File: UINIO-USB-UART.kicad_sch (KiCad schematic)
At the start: 32 parts, among them J1 Conn_01x08_Male, J2 Conn_01x04_Male, J3 Conn_01x07_Male, J4 Conn_01x06_Male, J5 Conn_01x04_Male, J6 Conn_01x07_Male, SW1 TP-33103, U1 CP2102, U2 CH343P

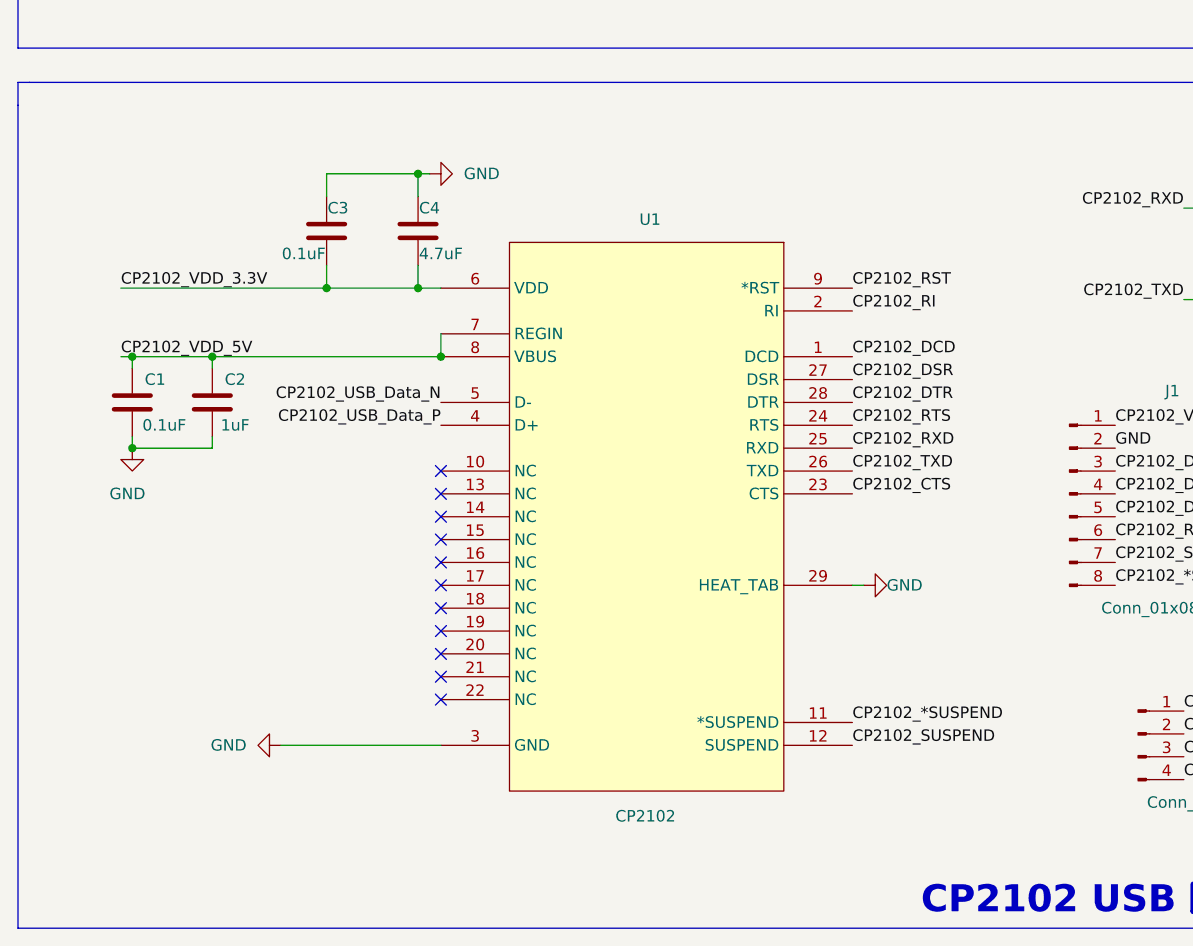
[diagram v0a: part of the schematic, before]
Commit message: Update libraries.
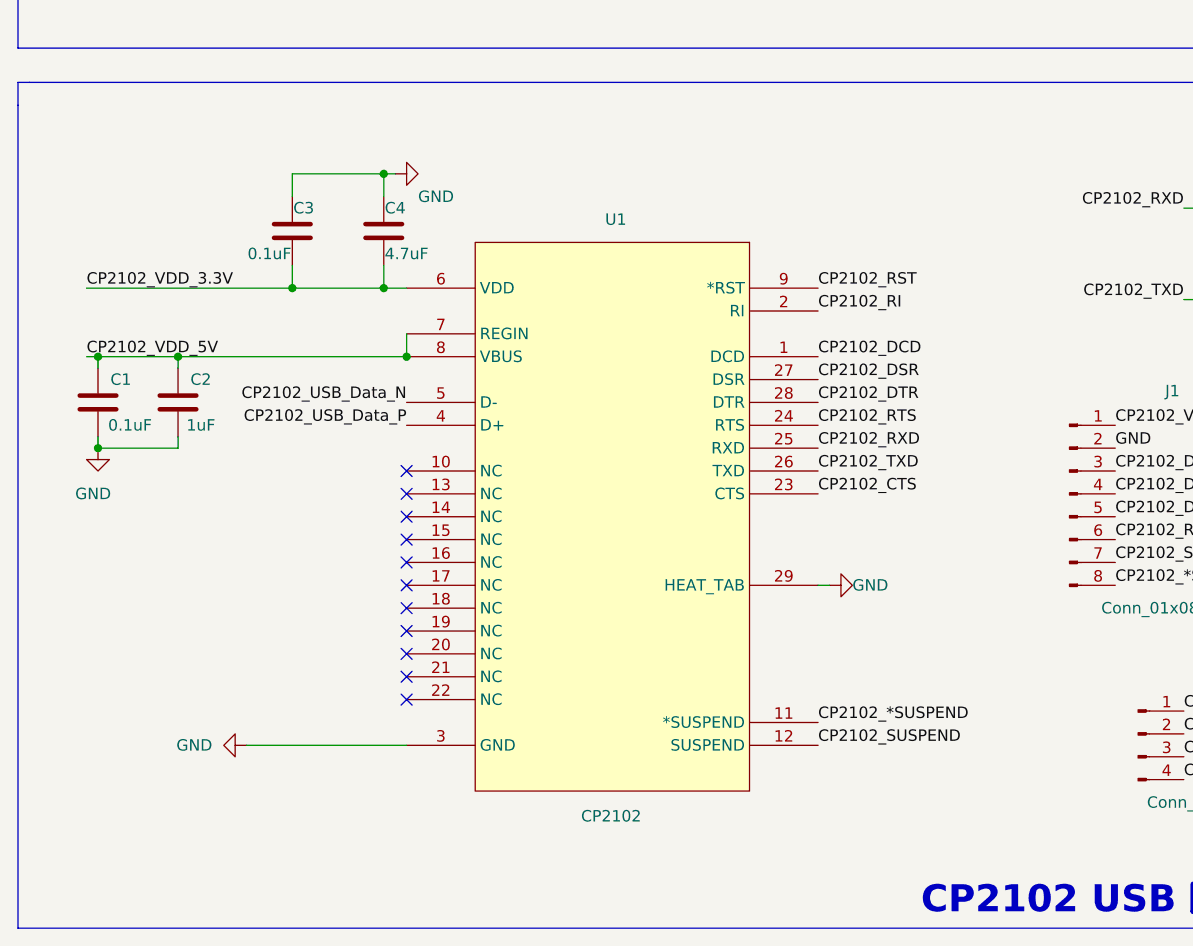
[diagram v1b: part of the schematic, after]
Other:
- moved on the sheet: C1, C2, C3, C4, U1
